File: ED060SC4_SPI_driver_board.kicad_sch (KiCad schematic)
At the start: 1 part, among them J1 ED060SC4

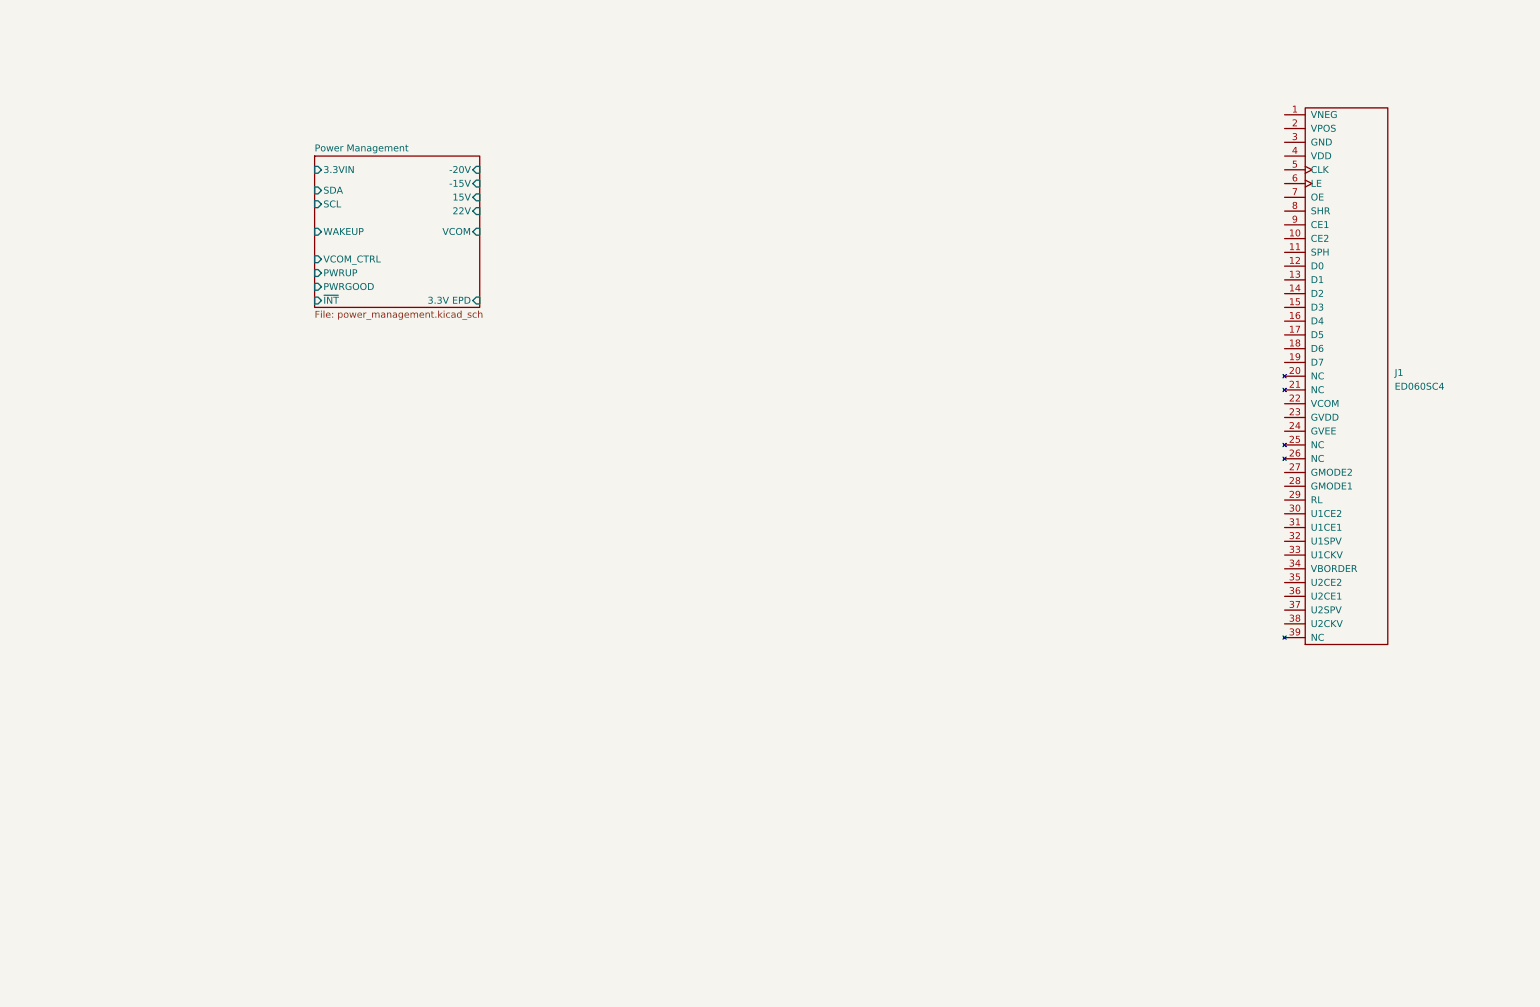
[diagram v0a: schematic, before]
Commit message: Full Schematic
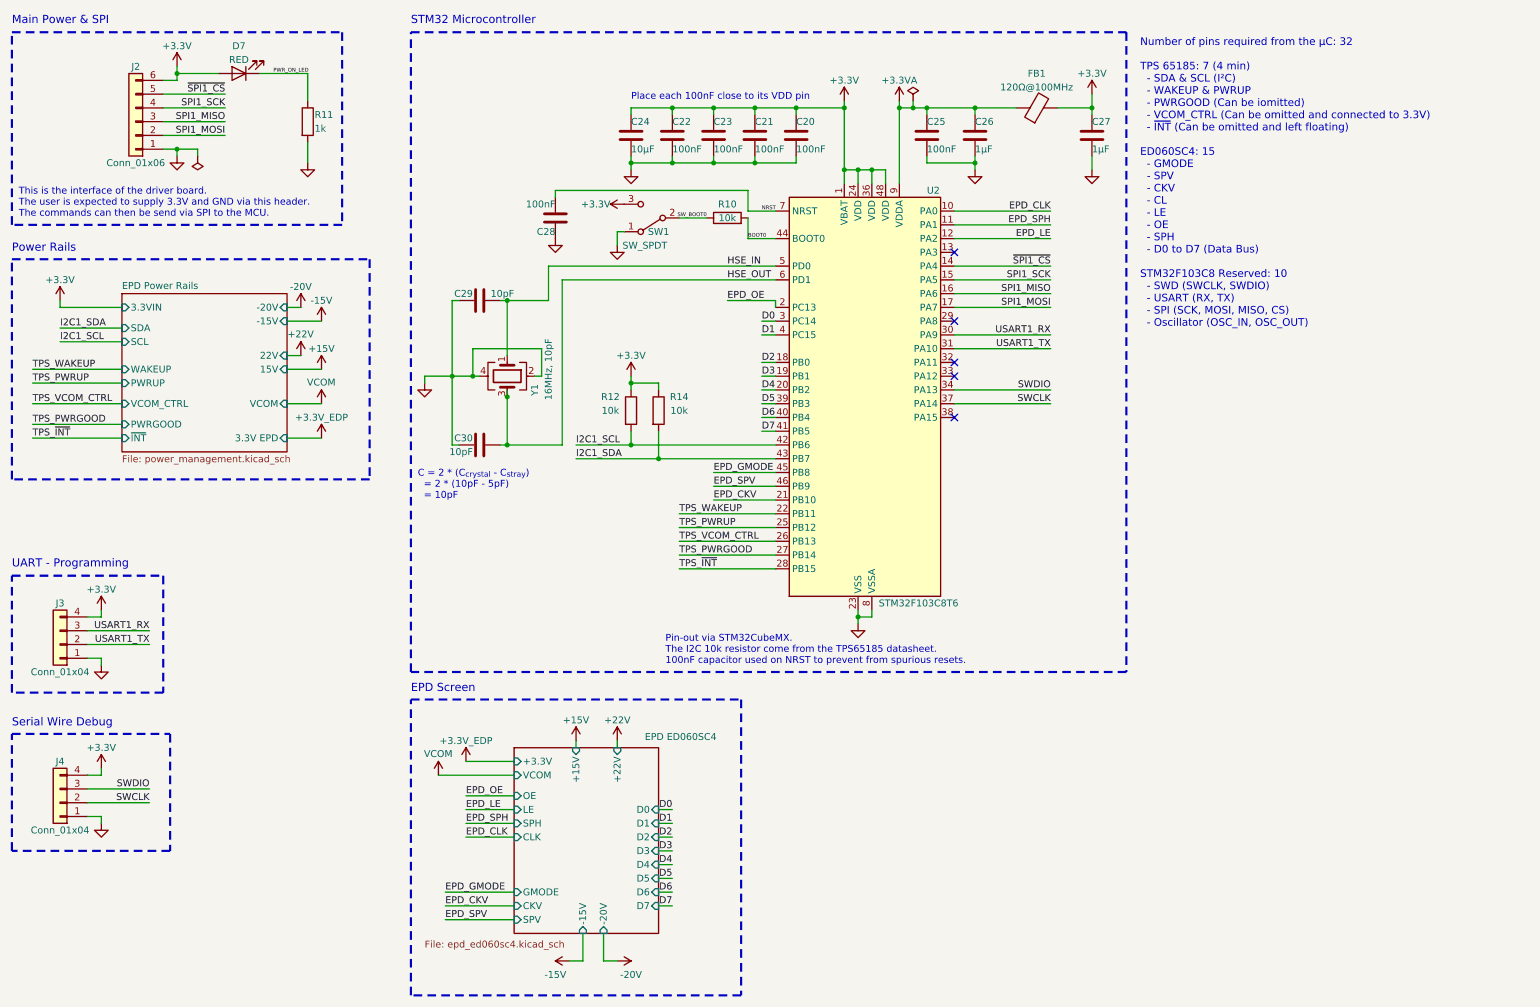
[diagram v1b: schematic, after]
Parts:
- removed J1: ED060SC4, symbol ED060SC4:ED060SC4
- added C20, C21, C22, C23, C25, C28: 100nF, symbol Device:C
- added C24: 10µF, symbol Device:C
- added C26, C27: 1µF, symbol Device:C
- added C29, C30: 10pF, symbol Device:C
- added D7: RED, symbol Device:LED
- added FB1: 120Ω@100MHz, symbol Device:FerriteBead
- added J2: Conn_01x06, symbol Connector_Generic:Conn_01x06
- added J3, J4: Conn_01x04, symbol Connector_Generic:Conn_01x04
- added R10, R12, R14: 10k, symbol Device:R
- added R11: 1k, symbol Device:R
- added SW1: SW_SPDT, symbol Switch:SW_SPDT
- added U2: STM32F103C8T6, Package_QFP:LQFP-48_7x7mm_P0.5mm, symbol MCU_ST_STM32F1:STM32F103C8Tx
- added Y1: 16MHz, 10pF, symbol Device:Crystal_GND24
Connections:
- new net +3.3V: C20.1, C21.1, C22.1, C23.1, C24.1, C27.1, D7.2 (A), FB1.2, J2.6 (Pin_6), J3.4 (Pin_4), J4.4 (Pin_4), R12.1, R14.1, SW1.3 (C), U2.1 (VBAT), U2.24 (VDD), U2.36 (VDD), U2.48 (VDD)
- new net +3.3VA: C25.1, C26.1, FB1.1, U2.9 (VDDA)
- new net BOOT0: R10.2, U2.44 (BOOT0)
- new net D0: U2.3 (PC14)
- new net D1: U2.4 (PC15)
- new net D2: U2.18 (PB0)
- new net D3: U2.19 (PB1)
- new net D4: U2.20 (PB2)
- new net D5: U2.39 (PB3)
- new net D6: U2.40 (PB4)
- new net D7: U2.41 (PB5)
- new net EPD_CKV: U2.21 (PB10)
- new net EPD_CLK: U2.10 (PA0)
- new net EPD_GMODE: U2.45 (PB8)
- new net EPD_LE: U2.12 (PA2)
- new net EPD_OE: U2.2 (PC13)
- new net EPD_SPH: U2.11 (PA1)
- new net EPD_SPV: U2.46 (PB9)
- new net GND: C20.2, C21.2, C22.2, C23.2, C24.2, C25.2, C26.2, C27.2, C28.1, C29.1, C30.1, J2.1 (Pin_1), J3.1 (Pin_1), J4.1 (Pin_1), R11.2, SW1.1 (A), U2.23 (VSS), U2.35 (VSS), U2.47 (VSS), U2.8 (VSSA), Y1.2, Y1.4
- new net HSE_IN: C29.2, U2.5 (PD0), Y1.1
- new net HSE_OUT: C30.2, U2.6 (PD1), Y1.3
- new net I2C1_SCL: R12.2, U2.42 (PB6)
- new net I2C1_SDA: R14.2, U2.43 (PB7)
- new net NRST: C28.2, U2.7 (NRST)
- new net PWR_ON_LED: D7.1 (K), R11.1
- new net SPI1_MISO: J2.3 (Pin_3), U2.16 (PA6)
- new net SPI1_MOSI: J2.2 (Pin_2), U2.17 (PA7)
- new net SPI1_SCK: J2.4 (Pin_4), U2.15 (PA5)
- new net SWCLK: J4.2 (Pin_2), U2.37 (PA14)
- new net SWDIO: J4.3 (Pin_3), U2.34 (PA13)
- new net SW_BOOT0: R10.1, SW1.2 (B)
- new net TPS_PWRGOOD: U2.27 (PB14)
- new net TPS_PWRUP: U2.25 (PB12)
- new net TPS_VCOM_CTRL: U2.26 (PB13)
- new net TPS_WAKEUP: U2.22 (PB11)
- new net TPS_~{INT}: U2.28 (PB15)
- new net USART1_RX: J3.3 (Pin_3), U2.30 (PA9)
- new net USART1_TX: J3.2 (Pin_2), U2.31 (PA10)
- new net ~{SPI1_CS}: J2.5 (Pin_5), U2.14 (PA4)
- no-connect marks 0 -> 5
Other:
- sheet Power Management renamed EPD Power Rails
- added sheet EPD ED060SC4 (epd_ed060sc4.kicad_sch)
- note added: "C = 2 * (C_{crystal} - C_{stray}) = 2 * (10pF - 5pF) = 10pF"
- note added: "EPD Screen"
- note added: "Main Power & SPI"
- note added: "Number of pins required from the µC: 32 TPS 65185: 7 (4 min) - SDA & SCL (I²C) - WAKEUP & PWRUP - PWRGOOD (Can be iomitted) - VCOM_CTRL (Can be omitted and connected to 3.3V) - ~{INT} (Can be omitted and left floating) ED060SC4: 15 - GMODE - SPV - CKV - CL - LE - OE - SPH - D0 to D7 (Data Bus) STM32F103C8 Reserved: 10 - SWD (SWCLK, SWDIO) - USART (RX, TX) - SPI (SCK, MOSI, MISO, CS) - Oscillator 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"
- note added: "Pin-out via STM32CubeMX. The I2C 10k resistor come from the TPS65185 datasheet. 100nF capacitor used on NRST to prevent from spurious resets."
- note added: "Place each 100nF close to its VDD pin"
- note added: "Power Rails"
- note added: "STM32 Microcontroller"
- note added: "Serial Wire Debug"
- note added: "This is the interface of the driver board. The user is expected to supply 3.3V and GND via this header. The commands can then be send via SPI to the MCU."
- note added: "UART - Programming"
- company: (none) -> hatrix
- title: (none) -> ED060SC4 SPI Driver Board
